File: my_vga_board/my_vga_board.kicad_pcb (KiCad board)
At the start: 4 copper layers, 23 parts, among them J1 Barrel_Jack, J2 L77HDE15SD1CH4F, U1 Pico, U2 LM7805_TO220

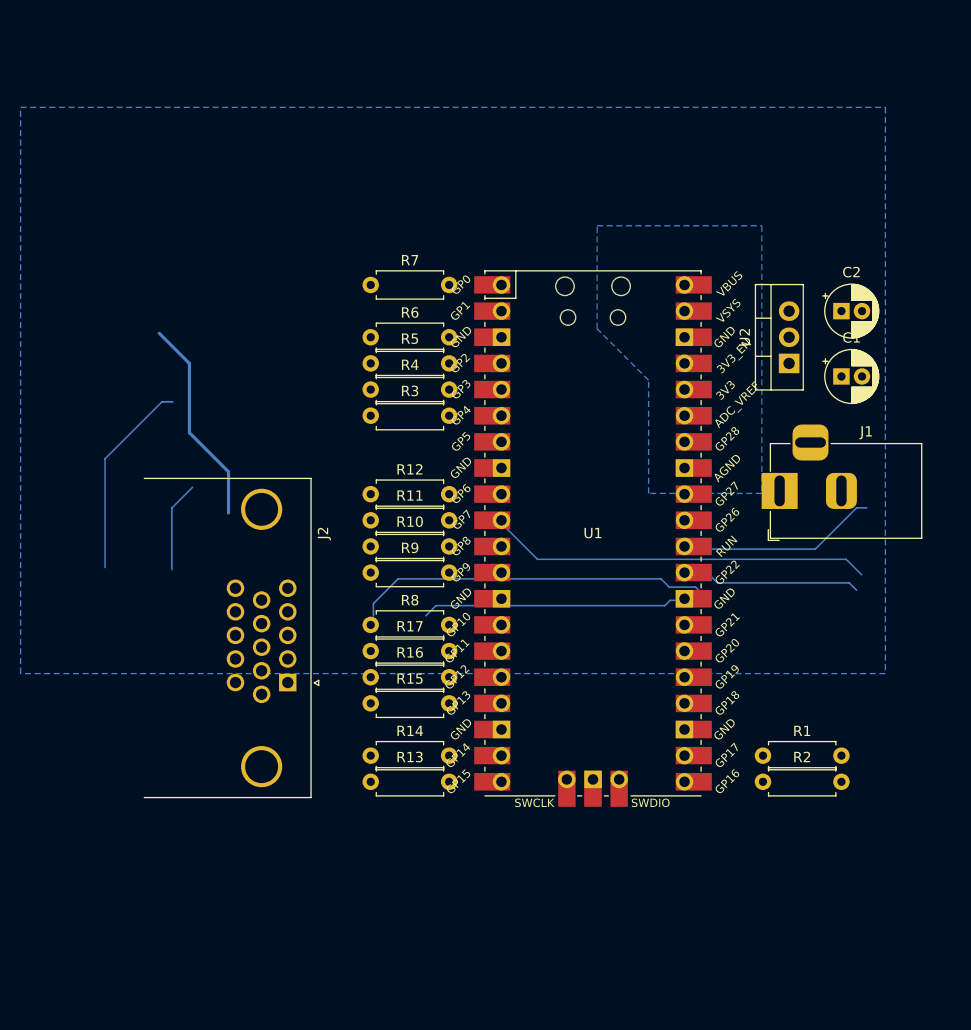
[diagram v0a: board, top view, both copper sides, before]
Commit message: adding tracks!  Neat
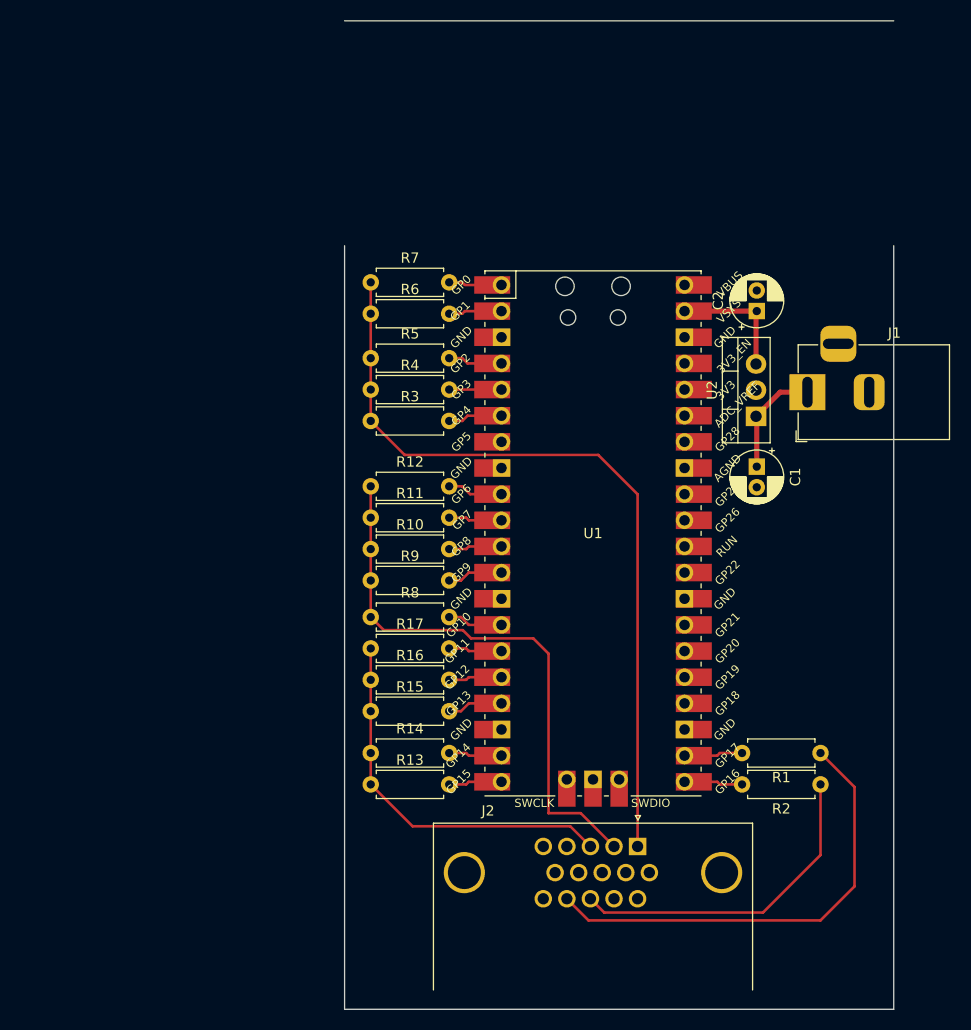
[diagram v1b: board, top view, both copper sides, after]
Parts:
- moved J2 55.4 mm to (149.6, 135.3), turned to 180 degrees
- moved C1 12.0 mm to (165.5, 84.4), turned to -90 degrees
- moved J1 9.97 mm to (170.4, 77.2)
- moved C2 8.22 mm to (165.5, 69.3), turned to 90 degrees
- moved U2 6.06 mm to (165.4, 79.5)
- moved R1 5.59 mm to (171.7, 112.2), turned to 180 degrees
- moved R2 5.59 mm to (171.7, 115.3), turned to 180 degrees
- moved R6 2.29 mm to (128.0, 69.5)
- moved R15 0.76 mm to (128.0, 108.2)
- moved R8 0.76 mm to (128.0, 99.0)
- moved R9 0.76 mm to (128.0, 95.5)
- moved R12 0.76 mm to (128.0, 86.3)
- moved R5 0.51 mm to (128.0, 73.9)
- moved R3 0.51 mm to (128.0, 80.0)
- moved R11 0.25 mm to (128.0, 89.4)
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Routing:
- net /VGA_R: track 0.00 -> 76.5 mm
- net GND: track 60.0 -> 0.00 mm
- net /VGA_G: track 0.00 -> 54.6 mm
- net /GPIO7: track 55.5 -> 5.19 mm
- net /VSYNC: track 0.00 -> 44.5 mm
- net /VGA_B: track 0.00 -> 37.0 mm
- net /HSYNC: track 0.00 -> 32.1 mm
- net /GPIO9: track 35.6 -> 5.40 mm
- net (no net): track 29.1 -> 0.00 mm
- net +5V: track 0.00 -> 12.2 mm
- net Net-(C1-Pad1): track 0.00 -> 10.9 mm
- net /GPIO17: track 0.00 -> 5.69 mm
- net /GPIO16: track 0.00 -> 5.69 mm
- net /GPIO13: track 0.00 -> 5.40 mm
- net /GPIO10: track 0.00 -> 5.40 mm
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- removed copper zone on B.Cu, net (none)
- removed copper zone on In1.Cu, net GND
- removed copper zone on In2.Cu, net GND
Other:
- board outline added: 53.3 x 96 mm
- rule pad_to_mask_clearance: 0.051 -> 0.0508
